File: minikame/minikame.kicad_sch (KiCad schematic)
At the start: 11 parts, among them J1 header3, J10 header3, J2 header3, J3 header3, J4 header3, J5 header, J6 header, J7 header3, J8 header3, J9 header3

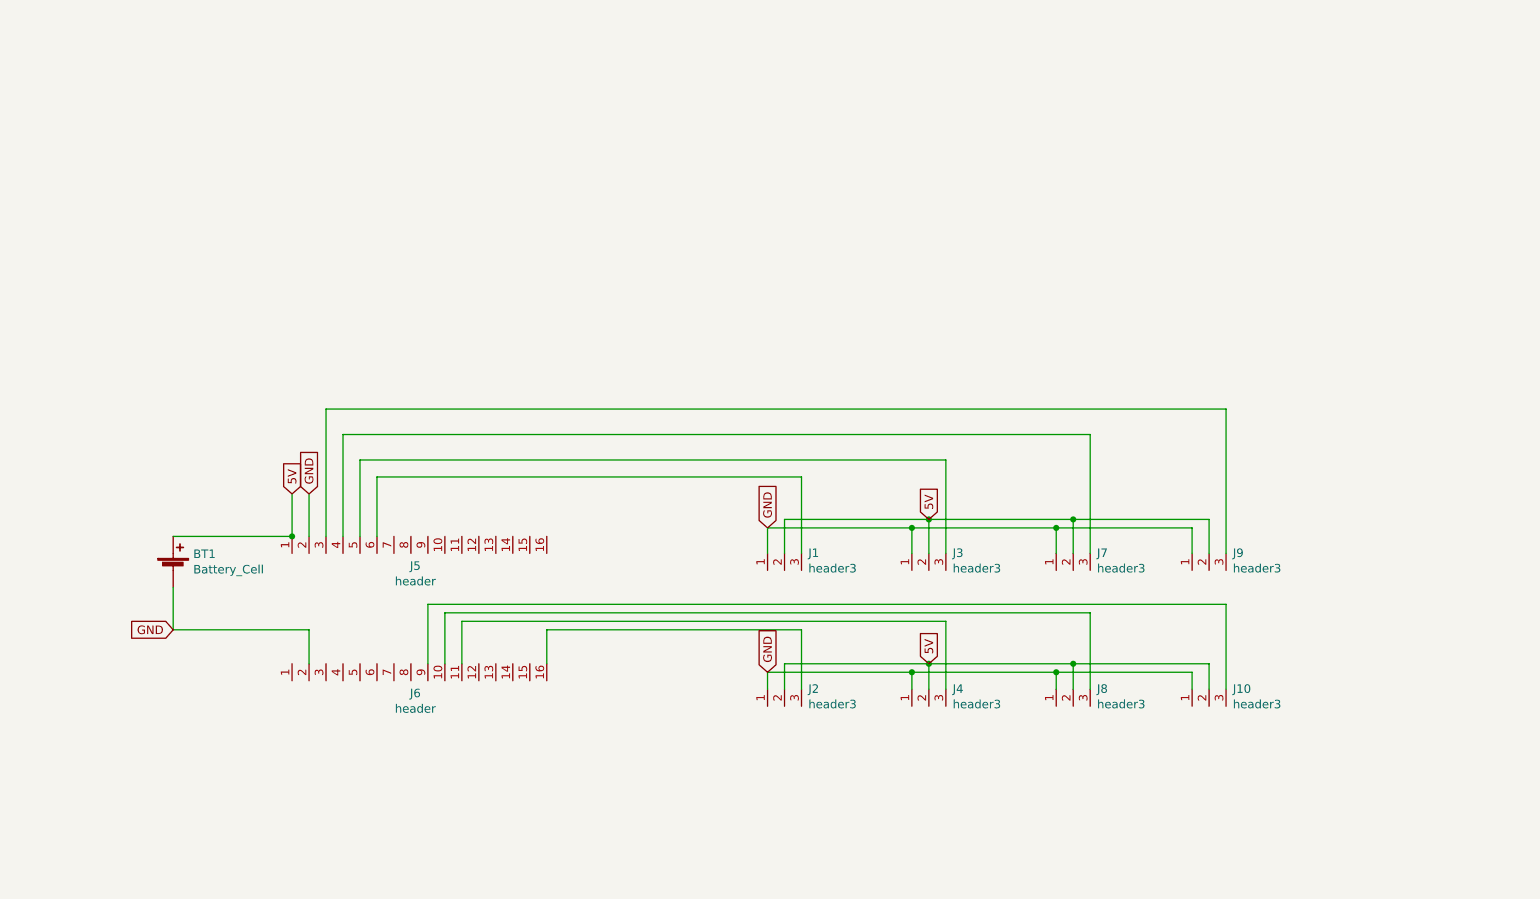
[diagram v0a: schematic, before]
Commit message: update
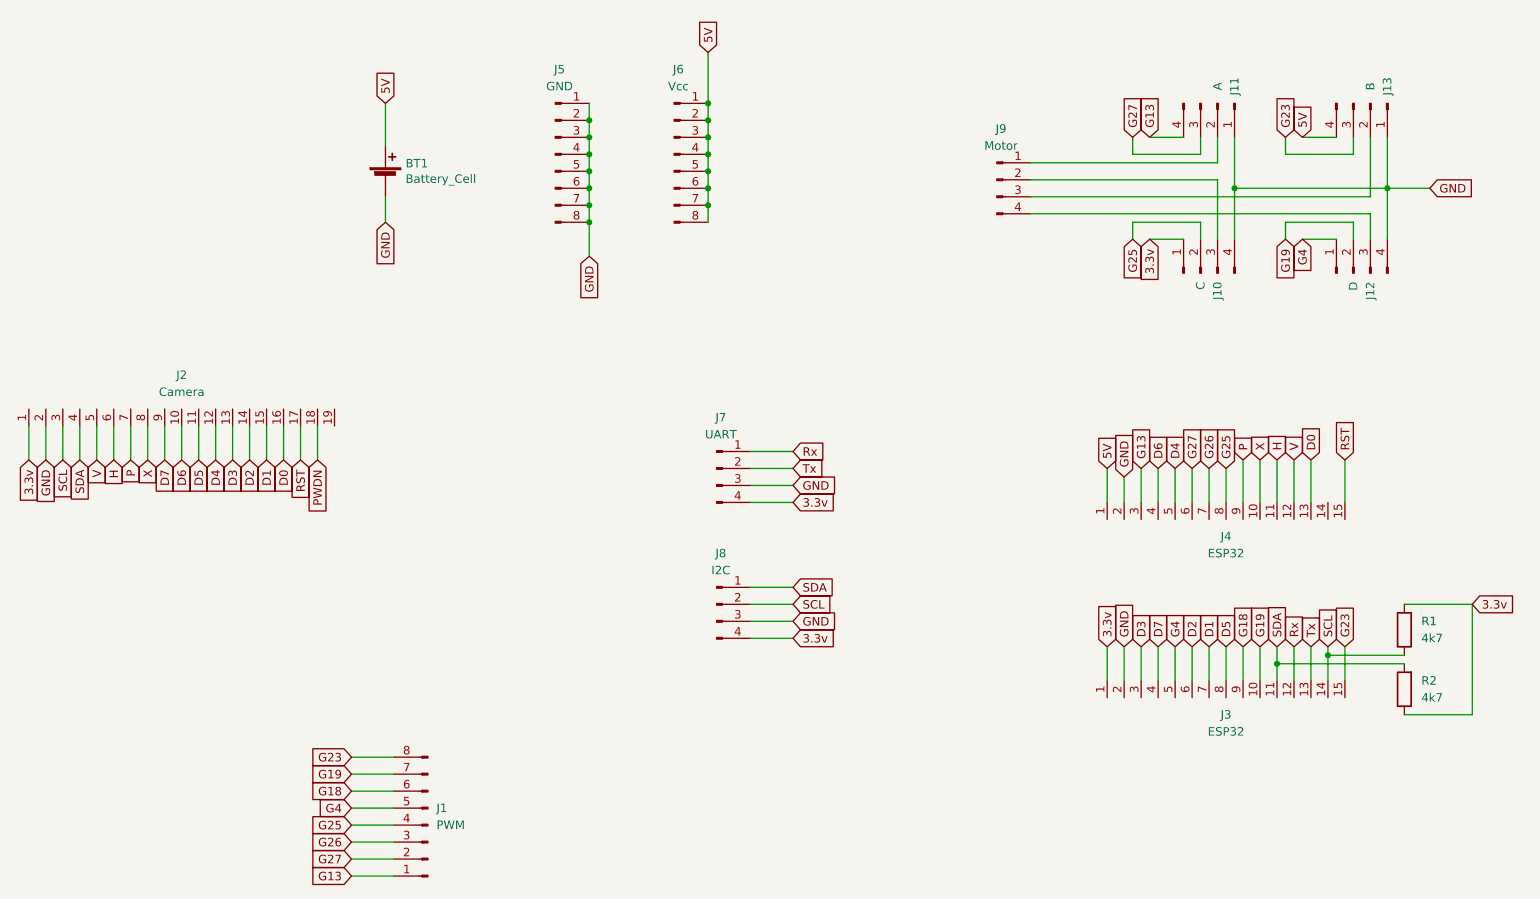
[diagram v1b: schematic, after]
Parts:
- removed J1, J10, J2, J3, J4, J7, J8, J9: header3, symbol minikame-rescue:header3-Header
- removed J5, J6: header, ESP32-footprints-Lib:PIN16, symbol minikame-rescue:header-Header
- added J1: PWM, symbol Connector:Conn_01x08_Male
- added J10: C, symbol Connector:Conn_01x04_Male
- added J11: A, symbol Connector:Conn_01x04_Male
- added J12: D, symbol Connector:Conn_01x04_Male
- added J13: B, symbol Connector:Conn_01x04_Male
- added J2: Camera, Connector_PinSocket_2.54mm:PinSocket_2x09_P2.54mm_Vertical, symbol Header:HDMI
- added J3, J4: ESP32, Connector_PinHeader_2.54mm:PinHeader_1x15_P2.54mm_Vertical, symbol Header:header15
- added J5: GND, symbol Connector:Conn_01x08_Male
- added J6: Vcc, symbol Connector:Conn_01x08_Male
- added J7: UART, symbol Connector:Conn_01x04_Male
- added J8: I2C, symbol Connector:Conn_01x04_Male
- added J9: Motor, symbol Connector:Conn_01x04_Male
- added R1, R2: 4k7, Resistor_SMD:R_0603_1608Metric, symbol Device:R
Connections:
- net 5V: now also J13.4 (Pin_4), J4.1, J6.1 (Pin_1), J6.2 (Pin_2), J6.3 (Pin_3), J6.4 (Pin_4), J6.5 (Pin_5), J6.6 (Pin_6), J6.7 (Pin_7), J6.8 (Pin_8)
- net GND: now also J10.4 (Pin_4), J11.1 (Pin_1), J12.4 (Pin_4), J13.1 (Pin_1), J2.2, J3.2, J4.2, J5.1 (Pin_1), J5.2 (Pin_2), J5.3 (Pin_3), J5.4 (Pin_4), J5.5 (Pin_5), J5.6 (Pin_6), J5.7 (Pin_7), J5.8 (Pin_8), J7.3 (Pin_3), J8.3 (Pin_3)
- new net: J11.2 (Pin_2), J9.1 (Pin_1)
- new net: J12.3 (Pin_3), J9.4 (Pin_4)
- new net: J13.2 (Pin_2), J9.3 (Pin_3)
- new net: J10.3 (Pin_3), J9.2 (Pin_2)
- new net 3.3v: J10.1 (Pin_1), J2.1, J3.1, J7.4 (Pin_4), J8.4 (Pin_4), R1.2, R2.1
- new net D0: J2.16, J4.13
- new net D1: J2.15, J3.7
- new net D2: J2.14, J3.6
- new net D3: J2.13, J3.3
- new net D4: J2.12, J4.5
- new net D5: J2.11, J3.8
- new net D6: J2.10, J4.4
- new net D7: J2.9, J3.4
- new net G13: J1.1 (Pin_1), J11.4 (Pin_4), J4.3
- new net G18: J1.6 (Pin_6), J3.9
- new net G19: J1.7 (Pin_7), J12.2 (Pin_2), J3.10
- new net G23: J1.8 (Pin_8), J13.3 (Pin_3), J3.15
- new net G25: J1.4 (Pin_4), J10.2 (Pin_2), J4.8
- new net G26: J1.3 (Pin_3), J4.7
- new net G27: J1.2 (Pin_2), J11.3 (Pin_3), J4.6
- new net G4: J1.5 (Pin_5), J12.1 (Pin_1), J3.5
- new net H: J2.6, J4.11
- new net P: J2.7, J4.9
- new net PWDN: J2.18
- new net RST: J2.17, J4.15
- new net Rx: J3.12, J7.1 (Pin_1)
- new net SCL: J2.3, J3.14, J8.2 (Pin_2), R1.1
- new net SDA: J2.4, J3.11, J8.1 (Pin_1), R2.2
- new net Tx: J3.13, J7.2 (Pin_2)
- new net V: J2.5, J4.12
- new net X: J2.8, J4.10
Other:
- moved on the sheet: BT1

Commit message: save
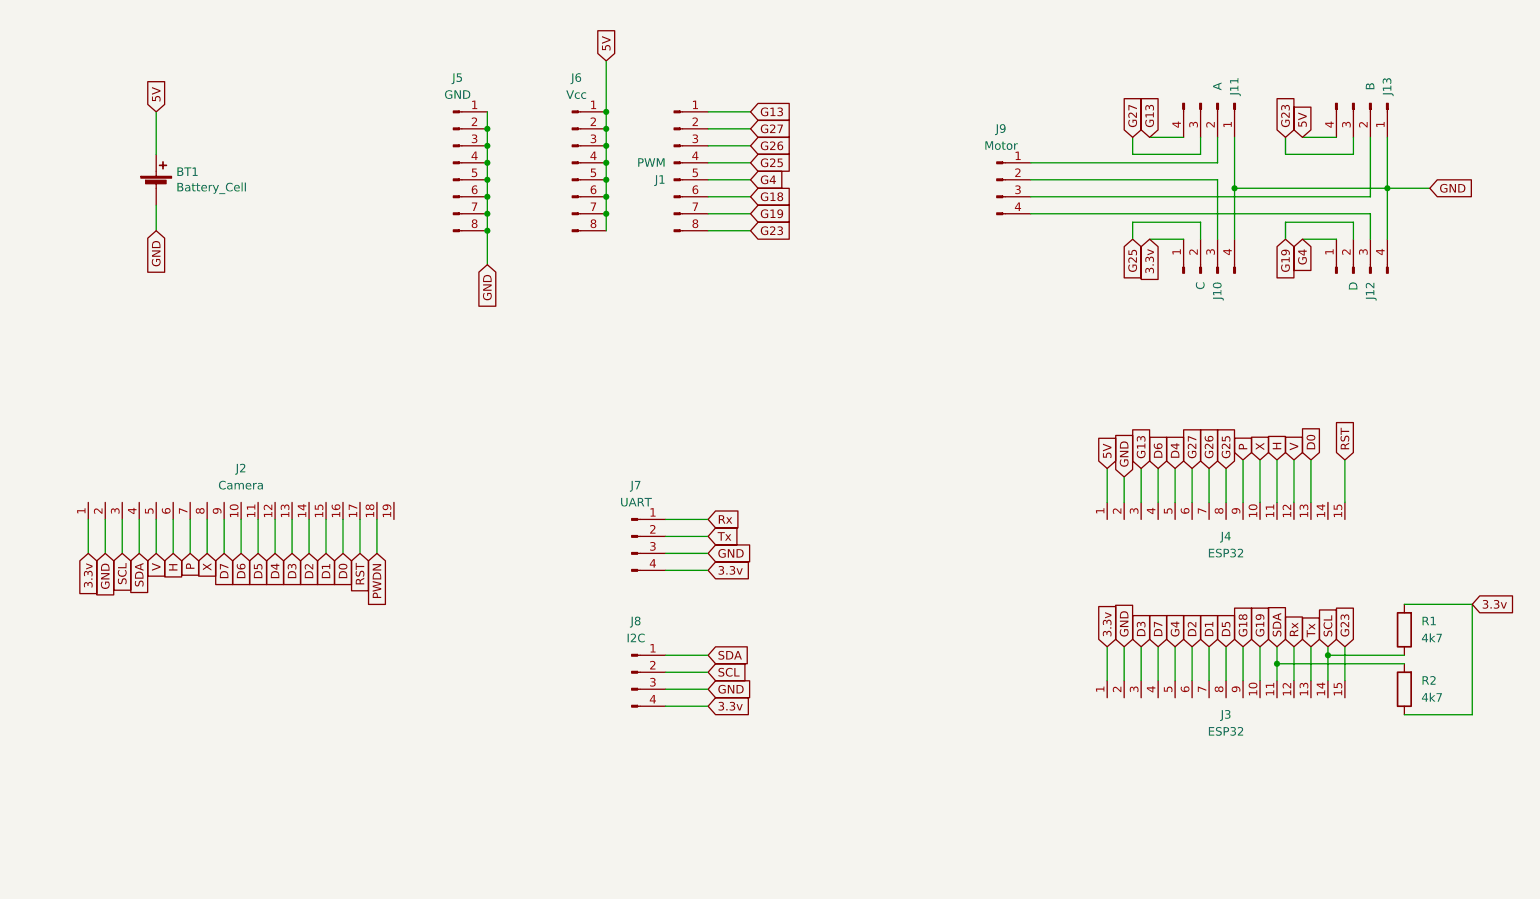
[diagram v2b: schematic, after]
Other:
- moved on the sheet: BT1, J1, J2, J5, J6, J7, J8
